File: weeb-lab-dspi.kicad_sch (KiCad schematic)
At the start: 55 parts, among them J1 SPDIF, J2 MONO RCA, J4 AudioJack3_Ground, Q1 BC846, U1 XIAO-RP2350-SMD, U2 MCP130-xxxDxTO, U3 CS8416-xNZ, U4 CS434x-xZZ

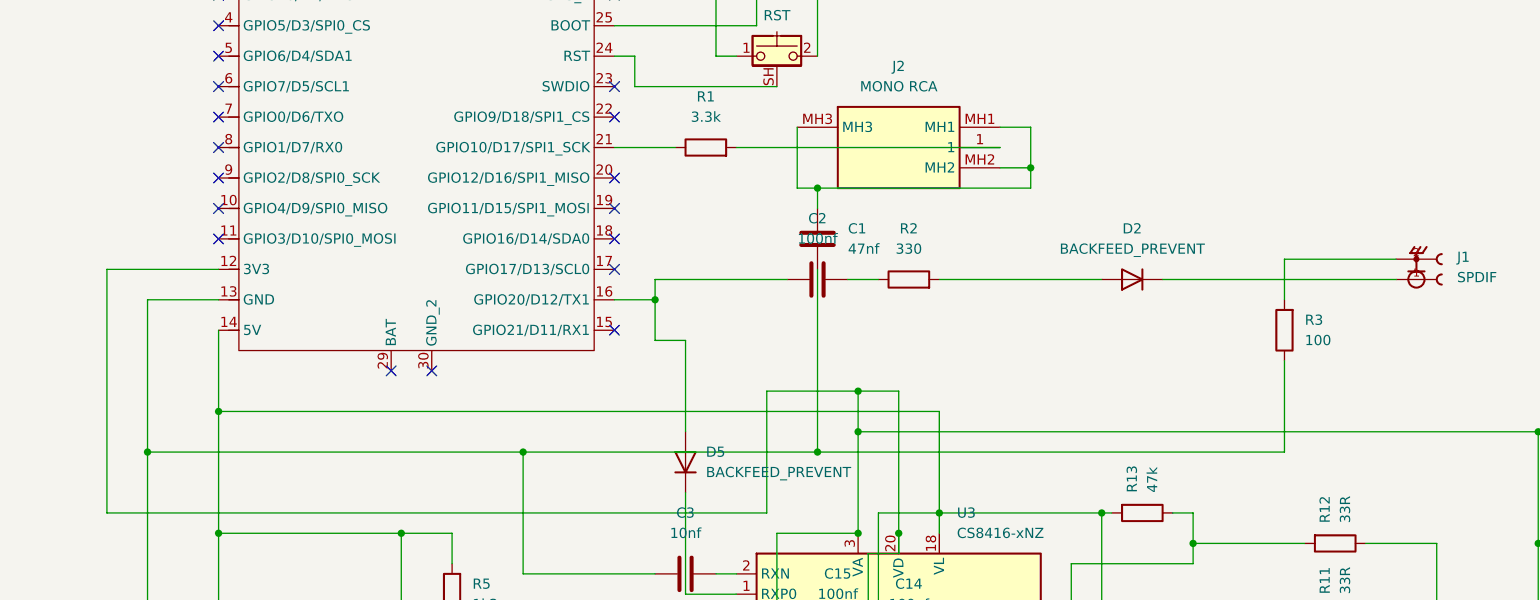
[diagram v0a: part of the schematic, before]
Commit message: Adding Labeling
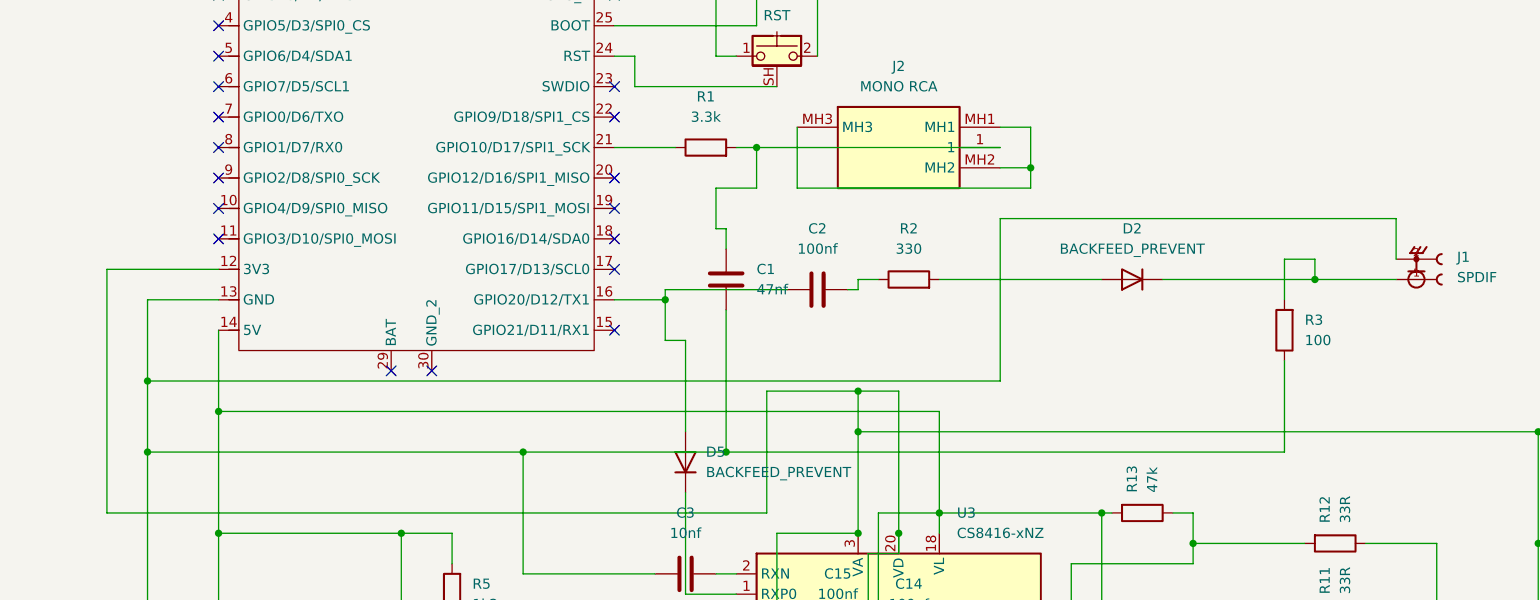
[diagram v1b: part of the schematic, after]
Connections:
- net GND: now also J1.2, J1.3, J1.4, J1.5
- net at J2.MH1, J2.MH2, J2.MH3: no longer C1.1
- net at D2.1 (K), J1.1: now also R3.2
- net at J2.1, R1.2: now also C1.1
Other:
- moved on the sheet: C1, C2
